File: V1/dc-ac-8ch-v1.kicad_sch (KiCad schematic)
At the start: 8 parts, among them J1 LOAD, J2 NEUTRAL, U1 MOC3031M

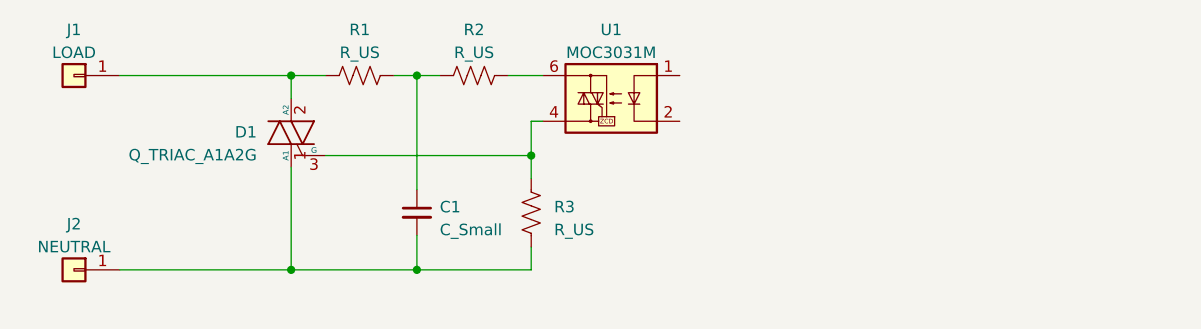
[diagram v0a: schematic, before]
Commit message: Circuit under dev
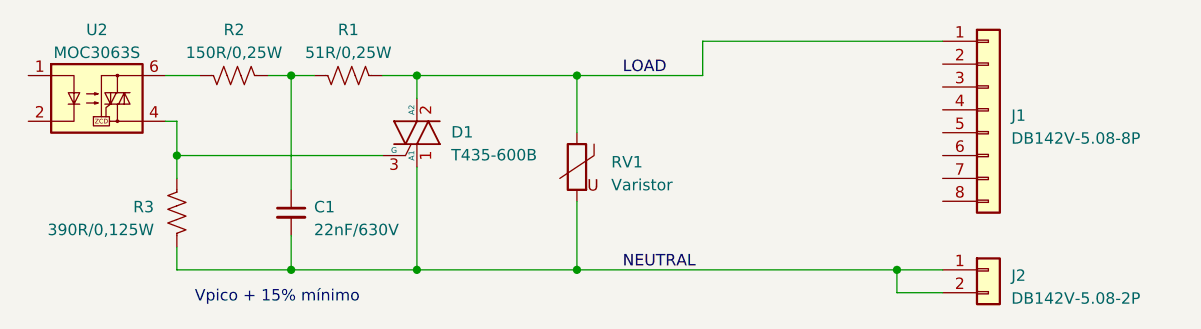
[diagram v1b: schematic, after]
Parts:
- removed J1: LOAD, symbol Connector_Generic:Conn_01x01
- removed J2: NEUTRAL, symbol Connector_Generic:Conn_01x01
- removed U1: MOC3031M, symbol Relay_SolidState:MOC3031M
- added J1: DB142V-5.08-8P, Tales:TerminalBlock_Dibo_DB142V-5.08-8P_1x08_P5.08mm_Vertical, symbol Connector_Generic:Conn_01x08
- added J2: DB142V-5.08-2P, Tales:TerminalBlock_Dibo_DB142V-5.08-2P_1x02_P5.08mm_Vertical, symbol Connector_Generic:Conn_01x02
- added RV1: Varistor, symbol Device:Varistor
- added U2: MOC3063S, Tales:SOP-6_6.6x9.15mm_P2.54mm, symbol Relay_SolidState:MOC3063M
- C1: value C_Small -> 22nF/630V; footprint (none) -> Tales:C_1206_3216Metric; JLCPCB BOM (none) -> 1; LCSC Part # (none) -> C318759; Mfr (none) -> Samsung Electro-Mechanics; Mfr Part # (none) -> CL31B223KHHNNNE; Package (none) -> 1206; Technology (none) -> X7R; Vendor (none) -> JLCPCB; Vendor Part # (none) -> C318759
- D1: value Q_TRIAC_A1A2G -> T435-600B; footprint (none) -> Tales:TO-252-2; JLCPCB BOM (none) -> 1; LCSC Part # (none) -> C145128; Mfr (none) -> STMicroelectronics; Mfr Part # (none) -> T435-600B-TR; Package (none) -> TO-252-2(DPAK); Technology (none) -> Snubberless; Vendor (none) -> JLCPCB; Vendor Part # (none) -> C145128
- R1: value R_US -> 51R/0,25W
- R2: value R_US -> 150R/0,25W
- R3: value R_US -> 390R/0,125W
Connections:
- net NEUTRAL: now reaches C1.2, D1.1 (A1), R3.2
- net NEUTRAL: now also J2.1 (Pin_1), J2.2 (Pin_2), RV1.2
- net LOAD: now reaches D1.2 (A2), R1.1
- net LOAD: now also J1.1 (Pin_1), RV1.1
- net at D1.3 (G), R3.1: now also U2.4
- net at R2.2: now also U2.6
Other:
- note added: "Vpico + 15% mínimo"
- moved on the sheet: C1, D1, R1, R2, R3
